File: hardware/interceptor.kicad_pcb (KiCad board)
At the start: 2 copper layers, 78.9 x 59.7 mm, 32 parts, among them IC1 ATMEGA1284P-P, P1 TAPEPORT, P2 CIA1, P3 KEYBOARD, P4 USER A, P5 USER B, P6 USB, SW1 RESET, SW2 BOOTLOADER, U1 7400, U2 ICL7660, U3 4520, U4 4051, U5 4051, U6 CD74HC22106, X1 16Mhz

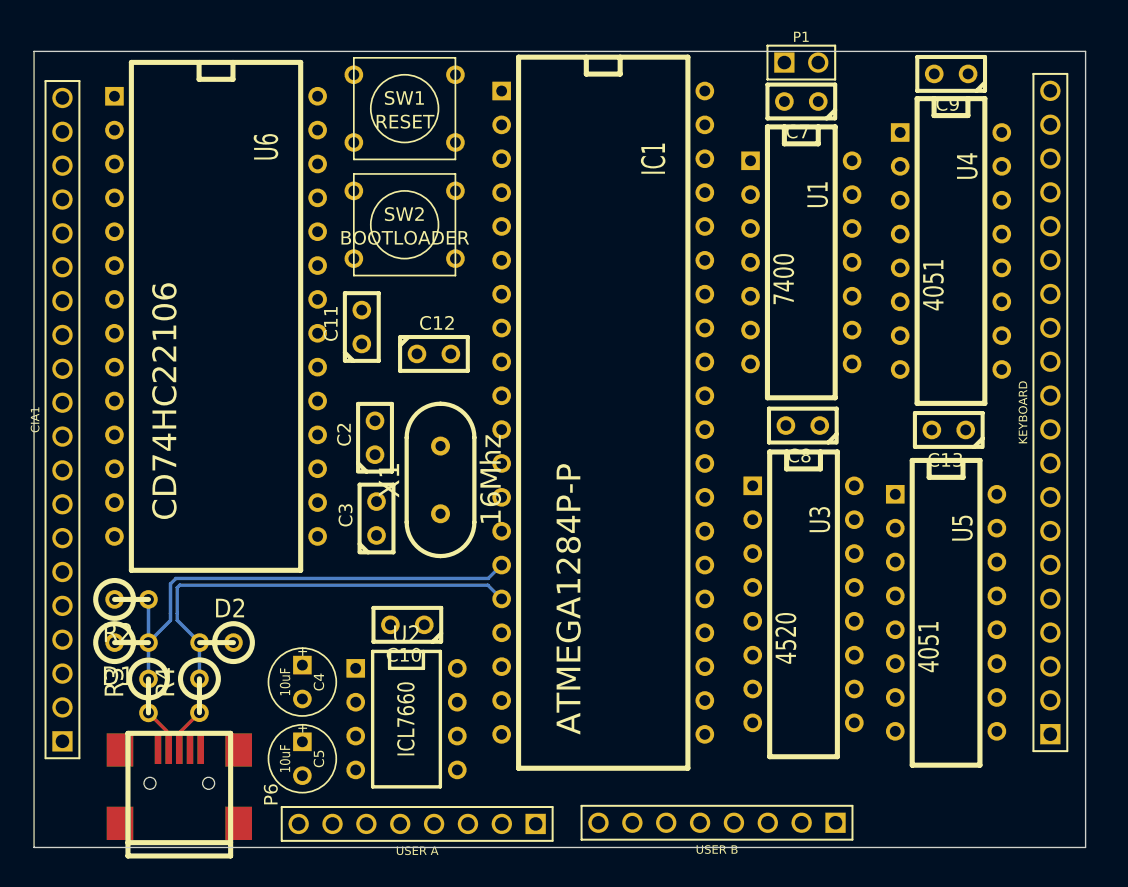
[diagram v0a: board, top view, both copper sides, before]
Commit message: Hardware: First serious draft of pcb layout
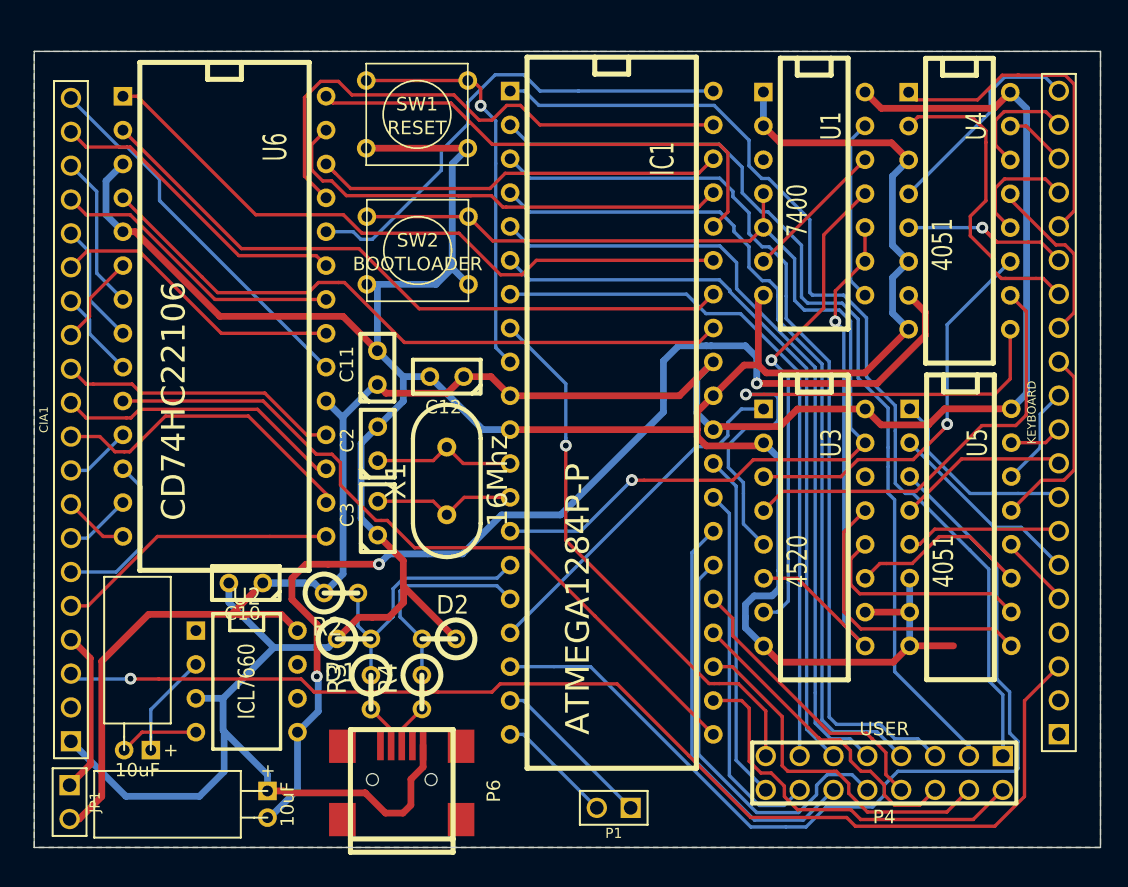
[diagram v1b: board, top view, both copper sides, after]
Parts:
- removed C13, C7, C8, C9: 100nF, C1
- removed P5: USER B, pinHeader-8x1
- added JP1: JUMPER, PIN_ARRAY_2X1, F.Cu at (16.2, 89.1)
- C4, C5: footprint C1V5 -> CR2H11W5H
- P4: value USER A -> USER; footprint pinHeader-8x1 -> pin_array_8x2
- moved P1 57.6 mm to (57.0, 89.6), turned to 180 degrees
- moved P4 35.2 mm to (77.3, 86.9)
- moved R3 16.7 mm to (38.8, 80.9)
- moved D1 16.7 mm to (37.5, 76.9)
- moved D2 16.7 mm to (43.9, 76.9)
- moved P6 16.7 mm to (41.1, 88.3)
- moved R4 16.7 mm to (42.6, 80.9)
- moved R2 15.7 mm to (36.5, 73.4)
- moved C4 13.4 mm to (21.3, 85.2), turned to 180 degrees
- moved C10 12.5 mm to (29.4, 72.7)
- moved U2 12.3 mm to (29.5, 80.1)
- moved U5 6.50 mm to (83.0, 68.5)
- moved U3 5.82 mm to (72.0, 68.5)
- moved U1 5.25 mm to (72.0, 43.5)
- moved C5 4.30 mm to (31.0, 89.3)
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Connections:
- P2 pad 4: VCC -> /EXTVCC
- P3 pad 4: VCC -> (no net)
- P4 pad 2: /UA1 -> /UB0
- P4 pad 3: /UA2 -> /UA1
- P4 pad 4: /UA3 -> /UB1
- P4 pad 5: /UA4 -> /UA2
- P4 pad 6: /UA5 -> /UB2
- P4 pad 7: /UA6 -> /UA3
- P4 pad 8: /UA7 -> /UB3
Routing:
- net GND: track 0.00 -> 280.5 mm
- net VCC: track 0.00 -> 155.8 mm
- net /~RESTORE: track 0.00 -> 88.5 mm, vias 0 -> 1
- net /VEE: track 0.00 -> 84.8 mm, vias 0 -> 3
- net /MR: track 0.00 -> 83.7 mm, vias 0 -> 1
- net /UA0: track 0.00 -> 76.7 mm
- net /UA1: track 0.00 -> 71.8 mm
- net /MD: track 0.00 -> 70.6 mm
- net /UA2: track 0.00 -> 69.6 mm
- net /UA3: track 0.00 -> 65.0 mm
- net /UA4: track 0.00 -> 60.0 mm
- net /~CPMR: track 0.00 -> 55.6 mm
- net /UA5: track 0.00 -> 55.6 mm
- net /UA6: track 0.00 -> 52.9 mm
- net /~CPS: track 0.00 -> 50.3 mm
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- added copper zone on B.Cu, net GND
- added copper zone on F.Cu, net GND
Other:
- board size 78.9 x 59.7 mm -> 80 x 59.7 mm
- net class Power added: clearance 0.254, trace_width 0.508, via_dia 0.889, via_drill 0.635
